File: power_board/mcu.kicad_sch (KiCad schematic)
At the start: 14 parts, among them U1 STM32L431KCUx

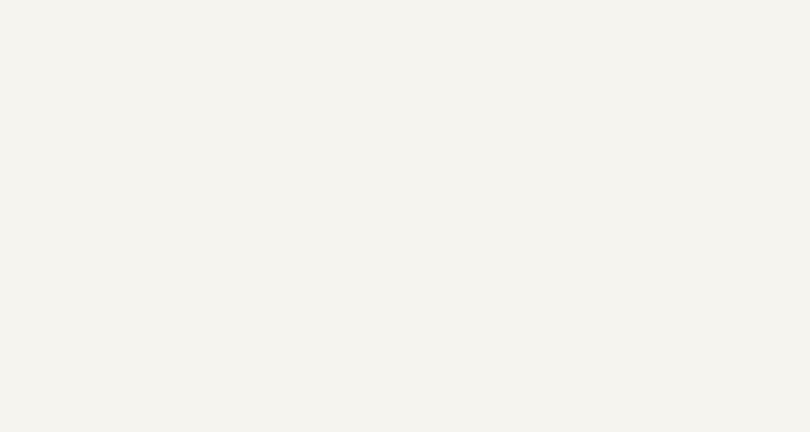
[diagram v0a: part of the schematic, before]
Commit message: All drc error solved
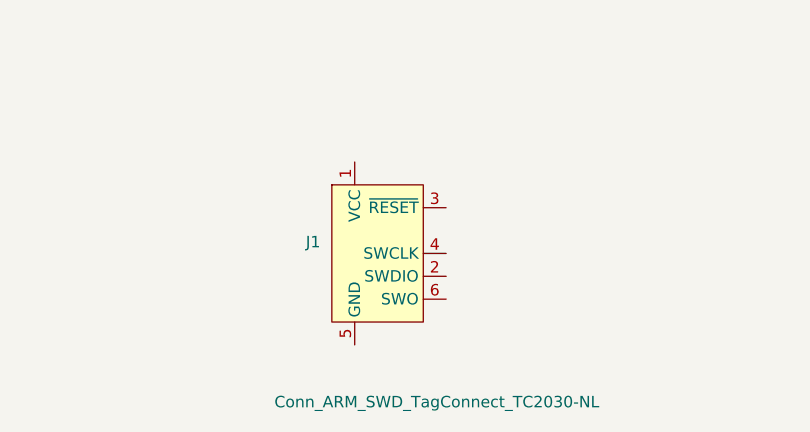
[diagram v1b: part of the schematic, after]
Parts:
- added J1: Conn_ARM_SWD_TagConnect_TC2030-NL, Connector:Tag-Connect_TC2030-IDC-NL_2x03_P1.27mm_Vertical, symbol Connector:Conn_ARM_SWD_TagConnect_TC2030-NL
- U1: footprint Package_DFN_QFN:QFN-32-1EP_5x5mm_P0.5mm_EP3.1x3.1mm_ThermalVias -> Package_DFN_QFN:QFN-32-1EP_5x5mm_P0.5mm_EP3.1x3.1mm
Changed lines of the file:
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@@
+	)
+	(symbol
+		(lib_id "Connector:Conn_ARM_SWD_TagConnect_TC2030-NL")
+		(at 44.45 134.62 0)
+		(unit 1)
+		(exclude_from_sim no)
+		(in_bom no)
+		(on_board yes)
+		(dnp no)
+		(property "Reference" "J1"
+			(at 38.1 133.3499 0)
+			(effects
+				(font
+					(size 1.27 1.27)
+				)
+				(justify right)
+			)
+		)
+		(property "Value" "Conn_ARM_SWD_TagConnect_TC2030-NL"
+			(at 69.088 151.13 0)
+			(effects
+				(font
+					(size 1.27 1.27)
+				)
+				(justify right)
+			)
+		)
+		(property "Footprint" "Connector:Tag-Connect_TC2030-IDC-NL_2x03_P1.27mm_Vertical"
+			(at 44.45 152.4 0)
+			(effects
+				(font
+					(size 1.27 1.27)
+				)
+				(hide yes)
+			)
+		)
+		(property "Datasheet" "https://www.tag-connect.com/wp-content/uploads/bsk-pdf-manager/TC2030-CTX_1.pdf"
+			(at 44.45 149.86 0)
+			(effects
+				(font
+					(size 1.27 1.27)
+				)
+				(hide yes)
+			)
+		)
+		(property "Description" "Tag-Connect ARM Cortex SWD JTAG connector, 6 pin, no legs"
+			(at 44.45 134.62 0)
+			(effects
+				(font
+					(size 1.27 1.27)
+				)
+				(hide yes)
+			)
+		)
+		(pin "1"
+		)
+		(pin "5"
+		)
+		(pin "3"
+		)
+		(pin "4"
+		)
+		(pin "2"
+		)
+		(pin "6"
+		)
+		(instances
+			(project ""
+				(path "/c786dd1f-c97f-4c1e-a27a-ac5828b3c50c/e75be158-cf9b-4215-a6e9-9f80ecc0638d"
+					(reference "J1")
+					(unit 1)
+				)
+			)
+		)
 	)
 	(symbol
@@
 			)
 		)
-		(property "Footprint" "Package_DFN_QFN:QFN-32-1EP_5x5mm_P0.5mm_EP3.1x3.1mm_ThermalVias"
+		(property "Footprint" "Package_DFN_QFN:QFN-32-1EP_5x5mm_P0.5mm_EP3.1x3.1mm"
 			(at 110.49 93.98 0)
 			(effects
